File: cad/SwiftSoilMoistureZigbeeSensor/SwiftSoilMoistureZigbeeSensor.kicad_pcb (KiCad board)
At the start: 2 copper layers, 83.8 x 22.9 mm, 13 parts, among them J1 Probe, J2 BAT, J3 ARM SWD, Q1 BSS84, SW1 Factory Reset, U1 TPS61221DCK, U2 E73-2G4M08S1C

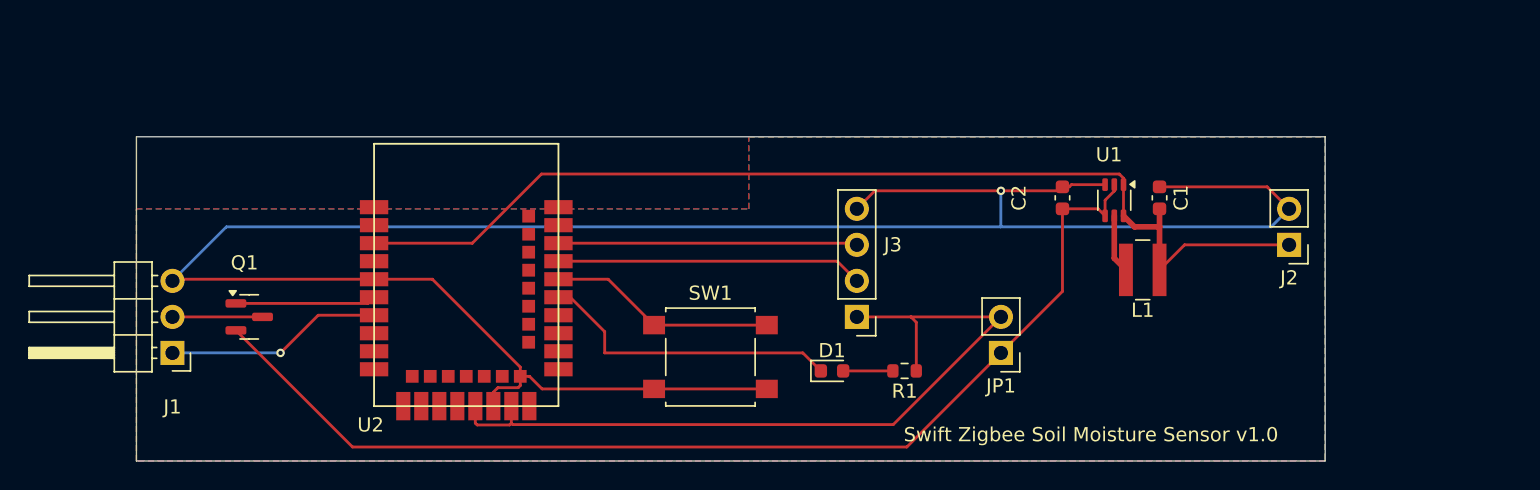
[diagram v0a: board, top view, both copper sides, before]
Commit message: PCB Version 1.1
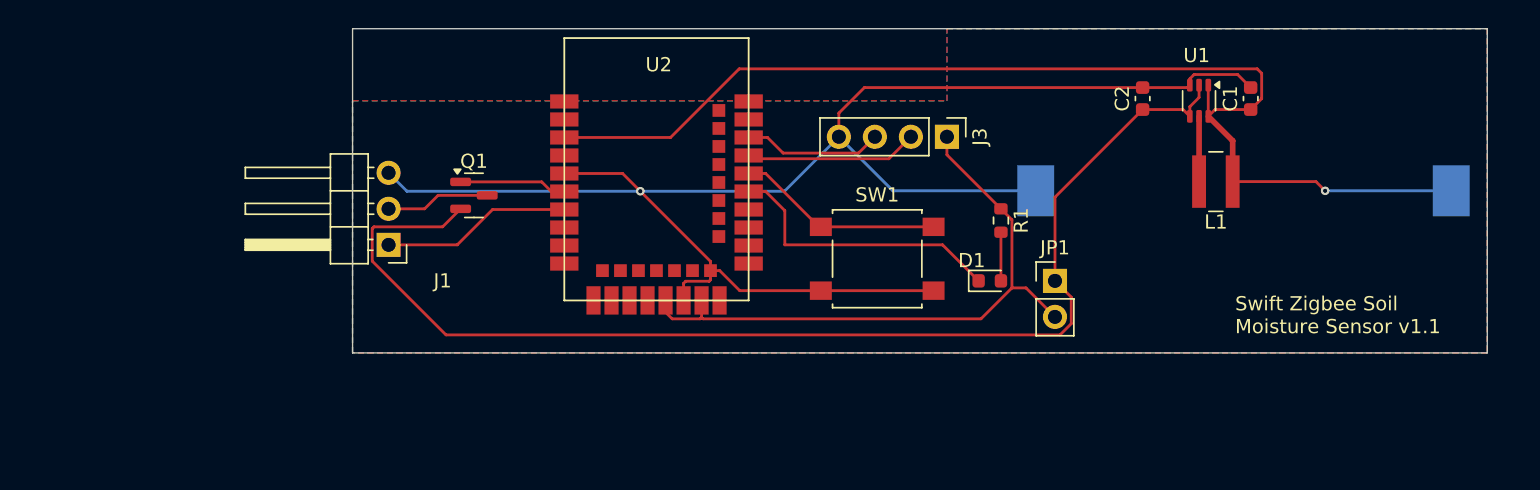
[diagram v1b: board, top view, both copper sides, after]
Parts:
- removed J2: BAT, Connector_PinHeader_2.54mm:PinHeader_1x02_P2.54mm_Vertical
- added BT1: CR2032, Battery:BatteryHolder_Keystone_1060_1x2032, B.Cu at (141.6, 54.6)
- moved Q1 18.0 mm to (87.3, 54.9)
- moved J1 17.0 mm to (81.3, 58.4)
- moved U2 15.3 mm to (100.2, 53.3)
- moved J3 14.2 mm to (120.7, 50.8), turned to -90 degrees
- moved SW1 13.7 mm to (115.7, 59.4)
- moved D1 12.8 mm to (123.7, 61.0)
- moved R1 12.6 mm to (124.5, 56.7), turned to -90 degrees
- moved C1 9.50 mm to (142.1, 48.1)
- moved U1 9.22 mm to (138.4, 48.3)
- moved C2 9.00 mm to (134.4, 48.1)
- moved L1 8.08 mm to (139.6, 54.0)
- moved JP1 6.35 mm to (128.3, 61.0), turned to 0 degrees
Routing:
- net GND: track 160.8 -> 115.6 mm
- net +3.3V: track 56.9 -> 44.1 mm
- net Net-(J3-SWDCLK): track 21.3 -> 9.83 mm
- net Net-(J3-SWDIO): track 21.6 -> 12.2 mm
- net Net-(JP1-A): track 77.7 -> 85.0 mm
- net Net-(BT1-+): track 74.7 -> 80.6 mm, vias 0 -> 1
- net Net-(Q1-G): track 9.92 -> 7.59 mm
- net Net-(J1-Pin_1): track 15.3 -> 13.4 mm, vias 1 -> 0
- net Net-(D1-K): track 21.7 -> 20.2 mm
- net Net-(U2B-P0.24): track 16.0 -> 14.6 mm
- net Net-(J1-Pin_2): track 6.35 -> 7.35 mm
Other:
- board size 83.8 x 22.9 mm -> 80 x 22.9 mm
- board text added: "Swift Zigbee Soil Moisture Sensor v1.1"
- board text removed: "Swift Zigbee Soil Moisture Sensor v1.0"
